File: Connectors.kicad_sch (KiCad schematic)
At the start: 4 parts, among them J1 Conn_01x04_Pin, J2 Conn_01x04_Pin, J3 Conn_01x09_Pin, J4 Conn_02x03_Odd_Even

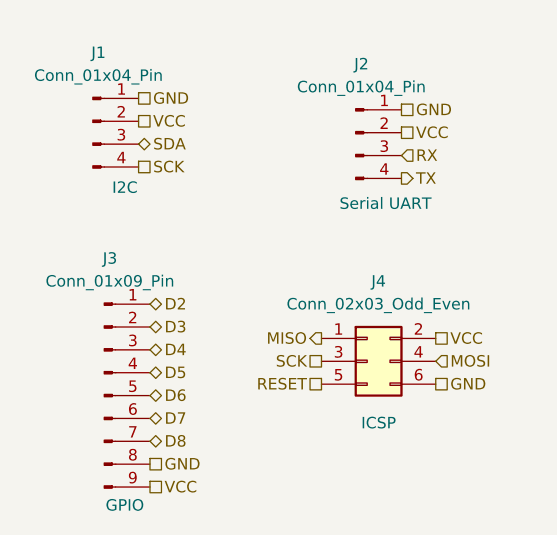
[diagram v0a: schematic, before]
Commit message: Completed comments
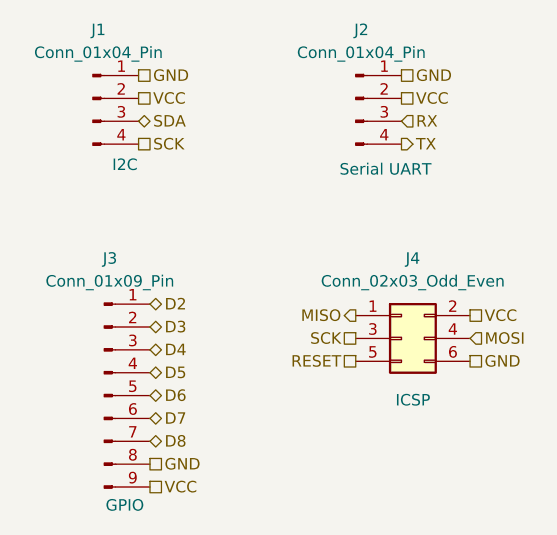
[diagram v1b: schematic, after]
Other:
- moved on the sheet: J1, J2, J4
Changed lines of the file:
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@@
 	(hierarchical_label "SDA"
 		(shape bidirectional)
-		(at 116.84 100.33 0)
+		(at 116.84 97.79 0)
 		(effects
 			(font
@@
 	(hierarchical_label "RX"
 		(shape input)
-		(at 146.05 101.6 0)
+		(at 146.05 97.79 0)
 		(effects
 			(font
@@
 	(hierarchical_label "GND"
 		(shape passive)
+		(at 116.84 92.71 0)
+		(effects
+			(font
+				(size 1.27 1.27)
+			)
+			(justify left)
+		)
+	)
+	(hierarchical_label "D7"
+		(shape bidirectional)
+		(at 118.11 130.81 0)
+		(effects
+			(font
+				(size 1.27 1.27)
+			)
+			(justify left)
+		)
+	)
+	(hierarchical_label "D2"
+		(shape bidirectional)
+		(at 118.11 118.11 0)
+		(effects
+			(font
+				(size 1.27 1.27)
+			)
+			(justify left)
+		)
+	)
+	(hierarchical_label "D5"
+		(shape bidirectional)
+		(at 118.11 125.73 0)
+		(effects
+			(font
+				(size 1.27 1.27)
+			)
+			(justify left)
+		)
+	)
+	(hierarchical_label "VCC"
+		(shape passive)
 		(at 116.84 95.25 0)
-		(effects
-			(font
-				(size 1.27 1.27)
-			)
-			(justify left)
-		)
-	)
-	(hierarchical_label "D7"
-		(shape bidirectional)
-		(at 118.11 130.81 0)
-		(effects
-			(font
-				(size 1.27 1.27)
-			)
-			(justify left)
-		)
-	)
-	(hierarchical_label "D2"
-		(shape bidirectional)
-		(at 118.11 118.11 0)
-		(effects
-			(font
-				(size 1.27 1.27)
-			)
-			(justify left)
-		)
-	)
-	(hierarchical_label "D5"
-		(shape bidirectional)
-		(at 118.11 125.73 0)
-		(effects
-			(font
-				(size 1.27 1.27)
-			)
-			(justify left)
-		)
-	)
-	(hierarchical_label "VCC"
-		(shape passive)
-		(at 116.84 97.79 0)
 		(effects
 			(font
@@
 	(hierarchical_label "MISO"
 		(shape output)
-		(at 137.16 121.92 180)
+		(at 140.97 119.38 180)
 		(effects
 			(font
@@
 	(hierarchical_label "MOSI"
 		(shape input)
-		(at 149.86 124.46 0)
+		(at 153.67 121.92 0)
 		(effects
 			(font
@@
 	(hierarchical_label "VCC"
 		(shape passive)
-		(at 146.05 99.06 0)
+		(at 146.05 95.25 0)
 		(effects
 			(font
@@
 	(hierarchical_label "SCK"
 		(shape passive)
-		(at 116.84 102.87 0)
+		(at 116.84 100.33 0)
 		(effects
 			(font
@@
 	(hierarchical_label "GND"
 		(shape passive)
-		(at 146.05 96.52 0)
+		(at 146.05 92.71 0)
 		(effects
 			(font
@@
 	(hierarchical_label "VCC"
 		(shape passive)
-		(at 149.86 121.92 0)
+		(at 153.67 119.38 0)
 		(effects
 			(font
@@
 	(hierarchical_label "RESET"
 		(shape passive)
-		(at 137.16 127 180)
+		(at 140.97 124.46 180)
 		(effects
 			(font
@@
 	(hierarchical_label "TX"
 		(shape output)
-		(at 146.05 104.14 0)
+		(at 146.05 100.33 0)
 		(effects
 			(font
@@
 	(hierarchical_label "GND"
 		(shape passive)
-		(at 149.86 127 0)
+		(at 153.67 124.46 0)
 		(effects
 			(font
@@
 	(hierarchical_label "SCK"
 		(shape passive)
-		(at 137.16 124.46 180)
+		(at 140.97 121.92 180)
 		(effects
 			(font
@@
 	(symbol
 		(lib_id "Connector_Generic:Conn_02x03_Odd_Even")
-		(at 142.24 124.46 0)
+		(at 146.05 121.92 0)
 		(unit 1)
 		(body_style 1)
@@
 		(dnp no)
 		(property "Reference" "J4"
-			(at 143.51 115.57 0)
+			(at 147.32 113.03 0)
 			(show_name no)
 			(do_not_autoplace no)
@@
 		)
 		(property "Value" "Conn_02x03_Odd_Even"
-			(at 143.51 118.11 0)
+			(at 147.32 115.57 0)
 			(show_name no)
 			(do_not_autoplace no)
@@
 		)
 		(property "Footprint" "Connector_PinHeader_2.54mm:PinHeader_2x03_P2.54mm_Vertical"
-			(at 142.24 124.46 0)
+			(at 146.05 121.92 0)
 			(hide yes)
 			(show_name no)
@@
 		)
 		(property "Datasheet" ""
-			(at 142.24 124.46 0)
+			(at 146.05 121.92 0)
 			(hide yes)
 			(show_name no)
@@
 		)
 		(property "Description" "Generic connector, double row, 02x03, odd/even pin numbering scheme (row 1 odd numbers, row 2 even numbers), script generated (kicad-library-utils/schlib/autogen/connector/)"
-			(at 142.24 124.46 0)
+			(at 146.05 121.92 0)
 			(hide yes)
 			(show_name no)
@@
 		)
 		(property "Purpose" "ICSP"
-			(at 143.51 131.318 0)
+			(at 147.32 128.778 0)
 			(show_name no)
 			(do_not_autoplace no)
@@
 	(symbol
 		(lib_id "Connector:Conn_01x04_Pin")
-		(at 111.76 97.79 0)
+		(at 111.76 95.25 0)
 		(unit 1)
 		(body_style 1)
@@
 		(dnp no)
 		(property "Reference" "J1"
+			(at 112.395 87.63 0)
+			(show_name no)
+			(do_not_autoplace no)
+			(effects
+				(font
+					(size 1.27 1.27)
+				)
+			)
+		)
+		(property "Value" "Conn_01x04_Pin"
 			(at 112.395 90.17 0)
 			(show_name no)
@@
 			)
 		)
-		(property "Value" "Conn_01x04_Pin"
-			(at 112.395 92.71 0)
-			(show_name no)
-			(do_not_autoplace no)
-			(effects
-				(font
-					(size 1.27 1.27)
-				)
-			)
-		)
 		(property "Footprint" "Connector_PinHeader_2.54mm:PinHeader_1x04_P2.54mm_Vertical"
-			(at 111.76 97.79 0)
+			(at 111.76 95.25 0)
 			(hide yes)
 			(show_name yes)
@@
 		)
 		(property "Datasheet" ""
-			(at 111.76 97.79 0)
+			(at 111.76 95.25 0)
 			(hide yes)
 			(show_name no)
@@
 		)
 		(property "Description" "Generic connector, single row, 01x04, script generated"
-			(at 111.76 97.79 0)
+			(at 111.76 95.25 0)
 			(hide yes)
 			(show_name no)
@@
 		)
 		(property "Purpose" "I2C"
-			(at 115.316 105.156 0)
+			(at 115.316 102.616 0)
 			(show_name no)
 			(do_not_autoplace no)
@@
 	(symbol
 		(lib_id "Connector:Conn_01x04_Pin")
-		(at 140.97 99.06 0)
+		(at 140.97 95.25 0)
 		(unit 1)
 		(body_style 1)
@@
 		(dnp no)
 		(property "Reference" "J2"
-			(at 141.605 91.44 0)
+			(at 141.605 87.63 0)
 			(show_name no)
 			(do_not_autoplace no)
@@
 		)
 		(property "Value" "Conn_01x04_Pin"
-			(at 141.605 93.98 0)
+			(at 141.605 90.17 0)
 			(show_name no)
 			(do_not_autoplace no)
@@
 		)
 		(property "Footprint" "Connector_PinHeader_2.54mm:PinHeader_1x04_P2.54mm_Vertical"
-			(at 140.97 99.06 0)
+			(at 140.97 95.25 0)
 			(hide yes)
 			(show_name yes)
@@
 		)
 		(property "Datasheet" ""
-			(at 140.97 99.06 0)
+			(at 140.97 95.25 0)
 			(hide yes)
 			(show_name no)
@@
 		)
 		(property "Description" "Generic connector, single row, 01x04, script generated"
-			(at 140.97 99.06 0)
+			(at 140.97 95.25 0)
 			(hide yes)
 			(show_name no)
@@
 		)
 		(property "Purpose" "Serial UART"
-			(at 144.272 106.934 0)
-			(show_name no)
-			(do_not_autoplace no)
+			(at 144.272 103.124 0)
+			(show_name no)
+			(do_not_autoplace no)
